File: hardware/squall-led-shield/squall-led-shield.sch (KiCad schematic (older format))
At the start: 16 parts, among them J1 SQUALL_HEADER, Q1 Q_2NMOS

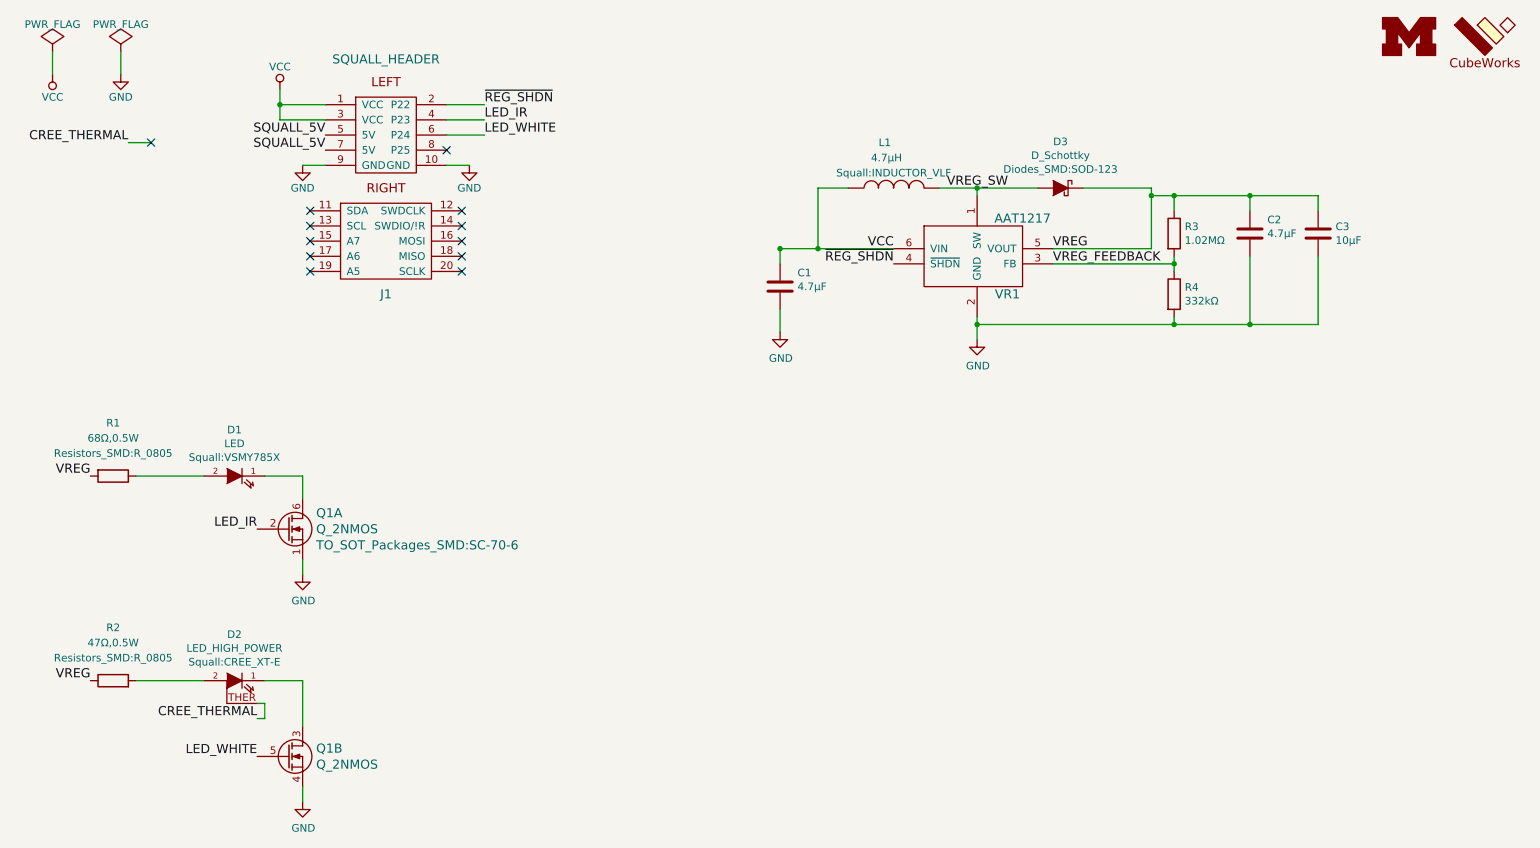
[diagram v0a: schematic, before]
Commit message: WIP: Add programming header
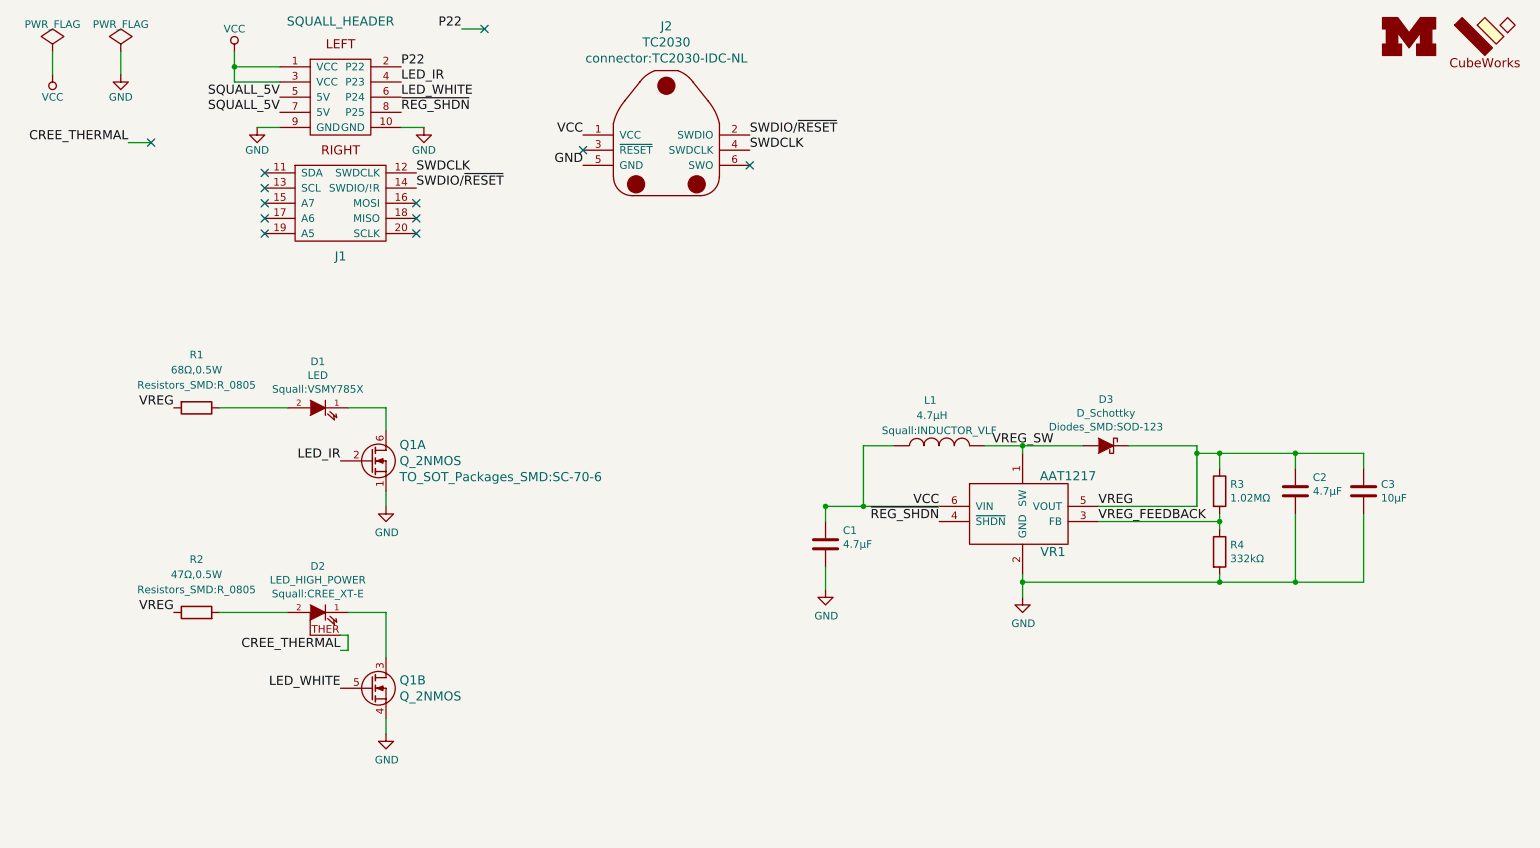
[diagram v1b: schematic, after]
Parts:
- added J2: TC2030, connector:TC2030-IDC-NL, symbol TC2030
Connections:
- net GND: now also J2.5 (GND)
- net VCC: now also J2.1 (VCC)
- net ~REG_SHDN: now also J1.8 (P25); no longer J1.2 (P22)
- net SWDCLK: now reaches J1.12 (SWDCLK)
- net SWDCLK: now also J2.4 (SWDCLK)
- net SWDIO/~RESET: now reaches J1.14 (SWDIO/!R)
- net SWDIO/~RESET: now also J2.2 (SWDIO)
- new net P22: J1.2 (P22)
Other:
- moved on the sheet: C1, C2, C3, D1, D2, D3, J1, L1, Q1A, Q1B, R1, R2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
